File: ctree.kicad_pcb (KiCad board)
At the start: 2 copper layers, 55 x 55 mm, 48 parts, among them IC1 ATMEGA328P-A, P1 CONN_02X03_PROG, Q1 IRLML6402, Q2 BC817, Q3 IRLML6402, Q4 IRLML6402, SW1 SMD_5.2x5.2, U1 MCP1624

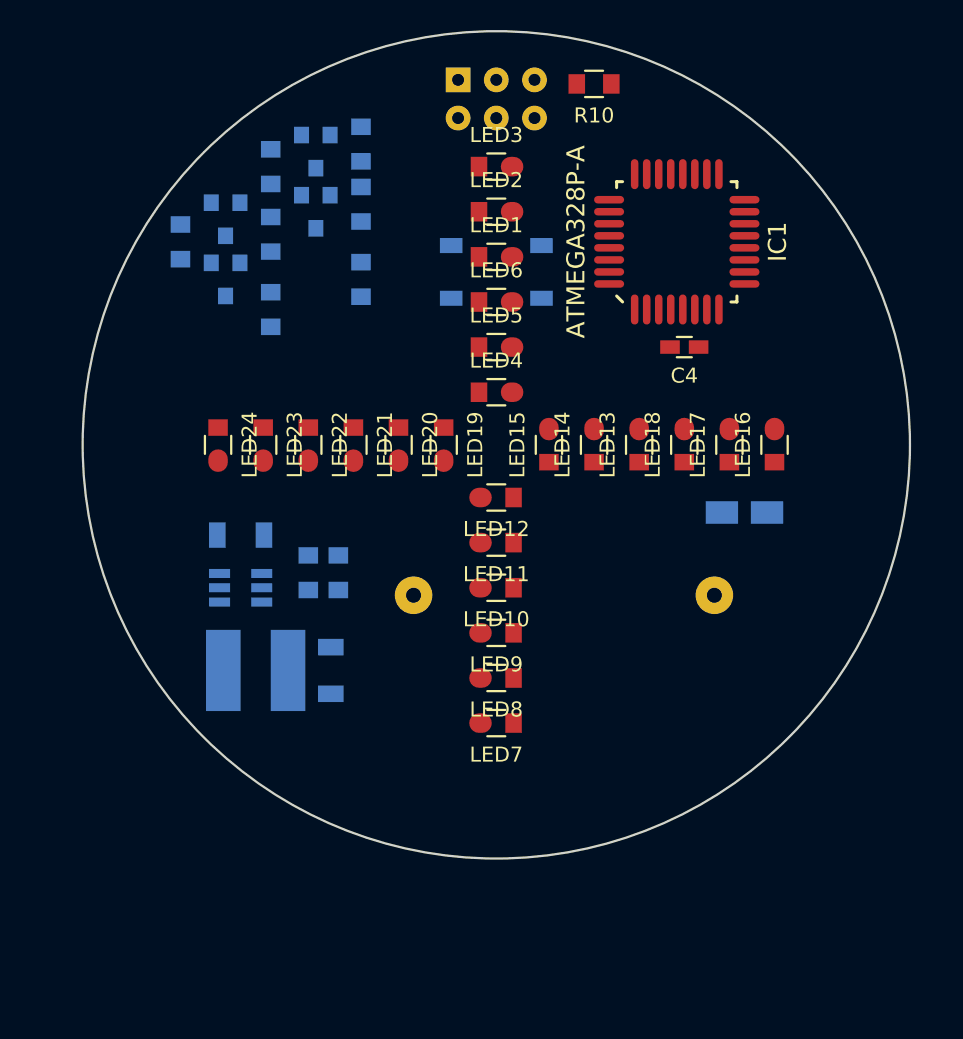
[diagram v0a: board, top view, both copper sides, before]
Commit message: PCB ready for fabrication.
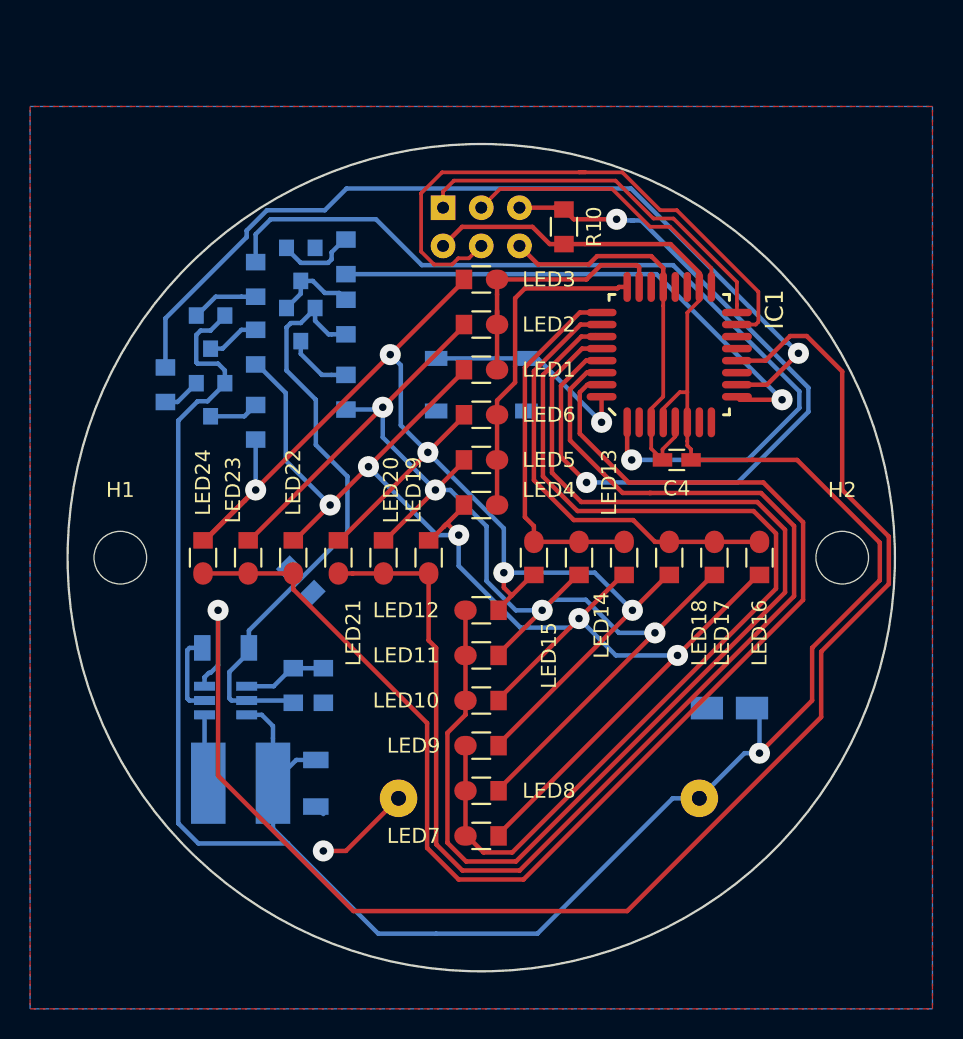
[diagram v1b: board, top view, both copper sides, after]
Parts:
- added H1: MountingHole, Mounting_Holes:MountingHole_3-5mm, F.Cu at (131.0, 65.0)
- added H2: MountingHole, Mounting_Holes:MountingHole_3-5mm, F.Cu at (179.0, 65.0)
- added H3: Logo, Attila:Logo, B.Cu at (174.0, 67.0)
- added RJ1: R_Jumper, Attila:RJ_0805_milling, B.Cu at (143.0, 66.5)
- moved BT1 13.5 mm to (157.5, 81.0)
- moved C3 13.0 mm to (171.5, 75.0)
- moved R10 9.71 mm to (160.5, 43.0), turned to 90 degrees
- moved R7 9.55 mm to (134.0, 53.5)
- moved P1 8.56 mm to (155.0, 43.0)
- moved Q3 8.06 mm to (137.0, 54.5)
- moved C1 7.57 mm to (144.0, 80.0)
- moved C2 7.57 mm to (138.0, 71.0)
- moved L1 7.57 mm to (139.0, 80.0)
- moved LED1 7.57 mm to (155.0, 52.5)
- moved LED10 7.57 mm to (155.0, 74.5)
- moved LED11 7.57 mm to (155.0, 71.5)
- moved LED12 7.57 mm to (155.0, 68.5)
- moved LED13 7.57 mm to (164.5, 65.0)
- moved LED14 7.57 mm to (161.5, 65.0)
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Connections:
- IC1 pad 25: /LED_C3 -> /LED_C5
- IC1 pad 26: /LED_C4 -> /LED_C6
- IC1 pad 27: /LED_C5 -> /LED_C3
- IC1 pad 28: /LED_C6 -> /LED_C4
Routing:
- net +BATT: track 0.00 -> 171.5 mm, vias 0 -> 1
- net /B_EN: track 0.00 -> 100.4 mm, vias 0 -> 1
- net /PWR_GREEN: track 0.00 -> 96.2 mm, vias 0 -> 5
- net /PWR_RED: track 0.00 -> 93.2 mm, vias 0 -> 5
- net /LED_C8: track 0.00 -> 88.4 mm
- net /PWR_BLUE: track 0.00 -> 86.7 mm, vias 0 -> 4
- net /LED_C7: track 0.00 -> 84.3 mm
- net /LED_C4: track 0.00 -> 77.9 mm
- net /LED_C3: track 0.00 -> 67.3 mm
- net /GREEN: track 0.00 -> 59.5 mm, vias 0 -> 1
- net /RED: track 0.00 -> 58.7 mm, vias 0 -> 1
- net /RESET: track 0.00 -> 52.9 mm, vias 0 -> 2
- net GND: track 0.00 -> 39.9 mm, vias 0 -> 1
- net +3V3: track 0.00 -> 39.7 mm
- net /MOSI: track 0.00 -> 39.7 mm
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- added copper zone on B.Cu, net GND
- added copper zone on F.Cu, net GND
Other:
- net class Default: clearance 0.2 -> 0.29; trace_width 0.25 -> 0.3; via_dia 0.6 -> 1.4; via_drill 0.4 -> 0.5
- rule trace_clearance: 0.2 -> 0.29
